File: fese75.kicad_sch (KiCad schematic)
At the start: 166 parts

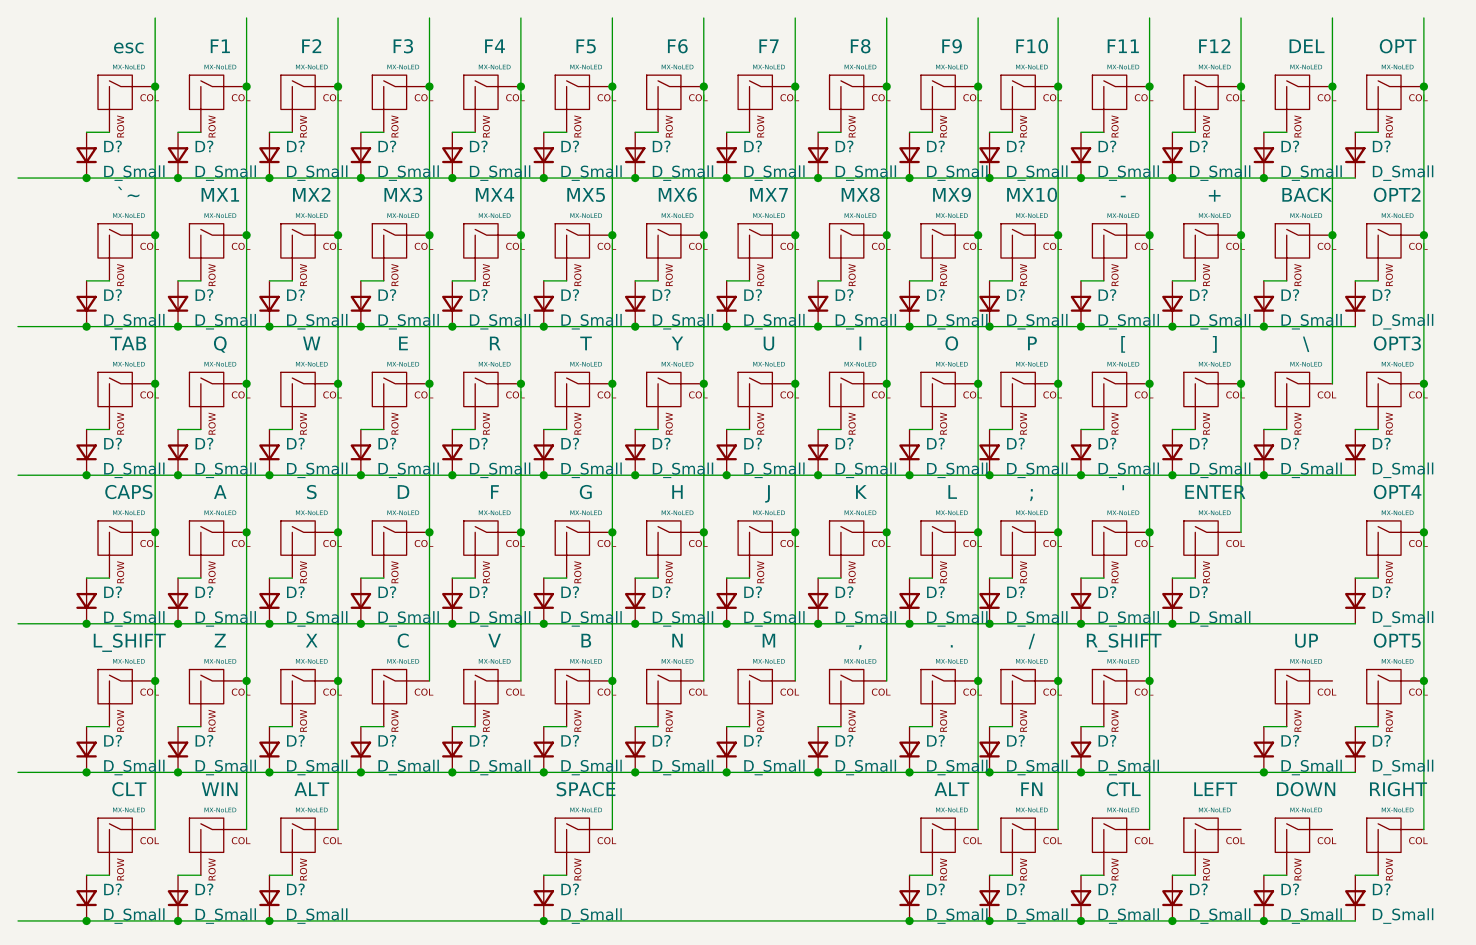
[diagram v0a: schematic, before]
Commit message: quick place component
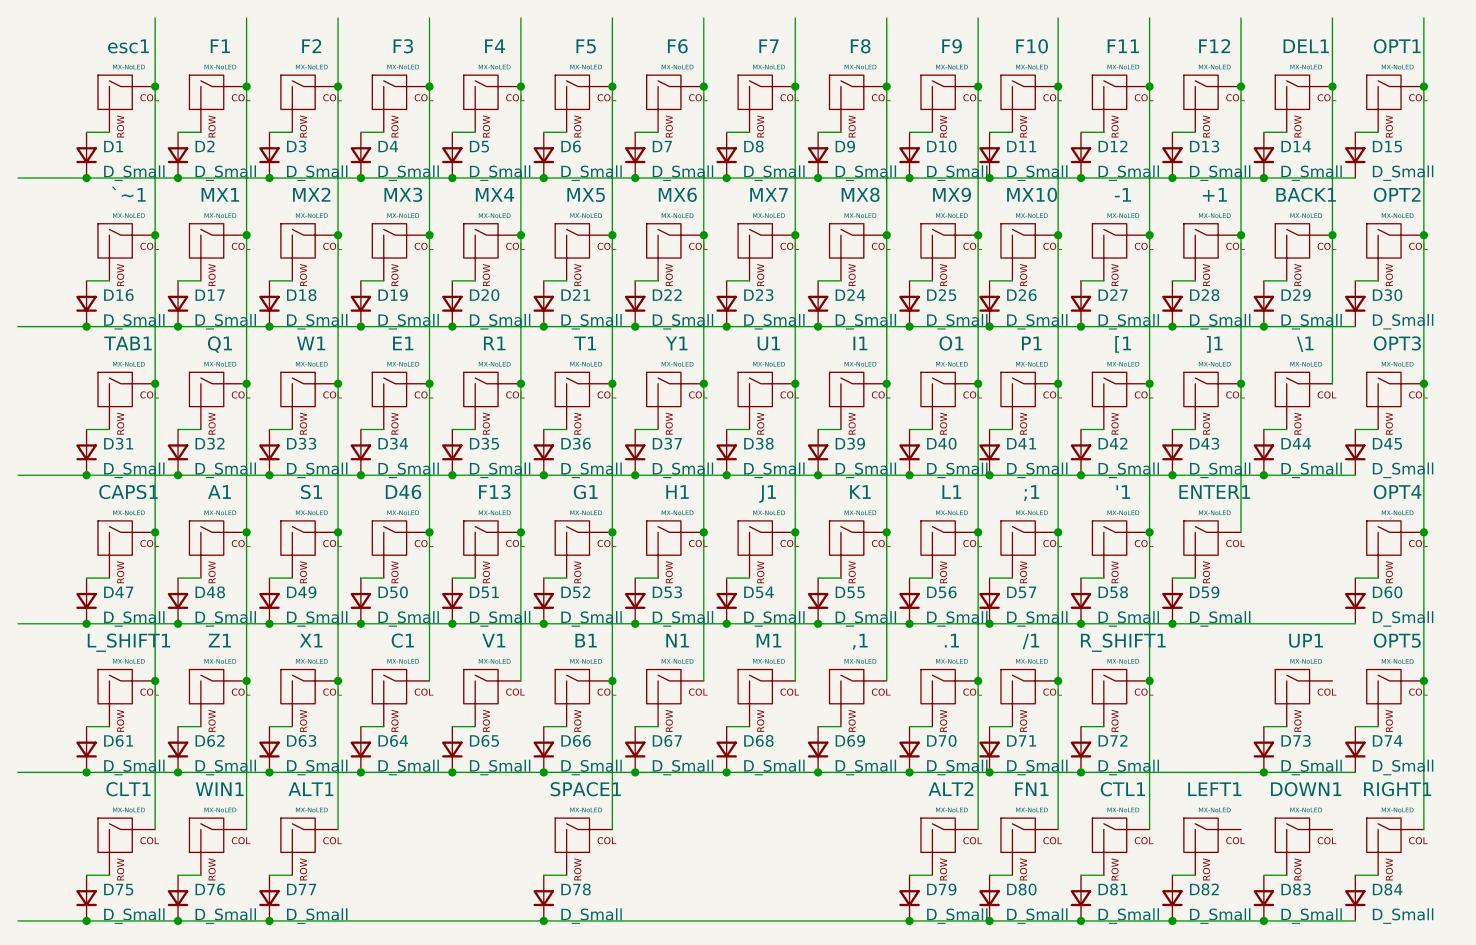
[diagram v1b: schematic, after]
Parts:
- '1: renamed from '; footprint Switch_Keyboard_Kailh:SW_Kailh_Choc_V1_1.00u -> Switch_Keyboard_Kailh:SW_Hotswap_Kailh_1.00u
- ,1: renamed from ,; footprint Mounting_Keyboard_Stabilizer:Stabilizer_Cherry_MX_6.25u -> Switch_Keyboard_Kailh:SW_Hotswap_Kailh_1.00u
- -1: renamed from -; footprint Switch_Keyboard_Kailh:SW_Kailh_Choc_V1_1.00u -> Switch_Keyboard_Kailh:SW_Hotswap_Kailh_1.00u
- .1: renamed from .; footprint Switch_Keyboard_Kailh:SW_Hotswap_Kailh_2.25u -> Switch_Keyboard_Kailh:SW_Hotswap_Kailh_1.00u
- /1: renamed from /; footprint Switch_Keyboard_Kailh:SW_Hotswap_Kailh_2.25u -> Switch_Keyboard_Kailh:SW_Hotswap_Kailh_1.00u
- ;1: renamed from ;; footprint Switch_Keyboard_Kailh:SW_Hotswap_Kailh_2.25u -> Switch_Keyboard_Kailh:SW_Hotswap_Kailh_1.00u
- A1: renamed from A; footprint Switch_Keyboard_Kailh:SW_Kailh_Choc_V1_1.00u -> Switch_Keyboard_Kailh:SW_Hotswap_Kailh_1.00u
- ALT2: renamed from ALT; footprint Switch_Keyboard_Kailh:SW_Hotswap_Kailh_2.25u -> Switch_Keyboard_Kailh:SW_Hotswap_Kailh_1.00u
- B1: renamed from B; footprint Switch_Keyboard_Kailh:SW_Hotswap_Kailh_2.25u -> Switch_Keyboard_Kailh:SW_Hotswap_Kailh_1.00u
- BACK1: renamed from BACK; footprint Mounting_Keyboard_Stabilizer:Stabilizer_Cherry_MX_6.25u -> Switch_Keyboard_Kailh:SW_Hotswap_Kailh_1.00u
- C1: renamed from C; footprint Mounting_Keyboard_Stabilizer:Stabilizer_Cherry_MX_6.25u -> Switch_Keyboard_Kailh:SW_Hotswap_Kailh_1.00u
- CAPS1: renamed from CAPS; footprint Switch_Keyboard_Kailh:SW_Hotswap_Kailh_2.25u -> Switch_Keyboard_Kailh:SW_Hotswap_Kailh_1.00u
- CLT1: renamed from CLT; footprint Switch_Keyboard_Kailh:SW_Hotswap_Kailh_2.25u -> Switch_Keyboard_Kailh:SW_Hotswap_Kailh_1.00u
- CTL1: renamed from CTL; footprint Switch_Keyboard_Kailh:SW_Kailh_Choc_V1_1.00u -> Switch_Keyboard_Kailh:SW_Hotswap_Kailh_1.00u
- D1, D10, D11, D12, D13, D14, D15, D16, D17, D18, D19, D2, D20, D21, D22, D23, D24, D25, D26, D27, D28, D29, D3, D30, D31, D32, D33, D34, D35, D36, D37, D38, D39, D4, D40, D41, D42, D43, D44, D45, D47, D48, D49, D5, D50, D51, D52, D53, D54, D55, D56, D57, D58, D59, D6, D60, D61, D62, D63, D64, D65, D66, D67, D68, D69, D7, D70, D71, D72, D73, D74, D75, D76, D77, D78, D79, D8, D80, D81, D82, D83, D84, D9: renamed from D?; footprint (none) -> Diode_SMD:D_0603_1608Metric_Pad1.05x0.95mm_HandSolder
- D46: renamed from D; footprint Mounting_Keyboard_Stabilizer:Stabilizer_Cherry_MX_6.25u -> Switch_Keyboard_Kailh:SW_Hotswap_Kailh_1.00u
- DEL1: renamed from DEL; footprint Mounting_Keyboard_Stabilizer:Stabilizer_Cherry_MX_6.25u -> Switch_Keyboard_Kailh:SW_Hotswap_Kailh_1.00u
- DOWN1: renamed from DOWN; footprint Mounting_Keyboard_Stabilizer:Stabilizer_Cherry_MX_6.25u -> Switch_Keyboard_Kailh:SW_Hotswap_Kailh_1.00u
- E1: renamed from E; footprint Mounting_Keyboard_Stabilizer:Stabilizer_Cherry_MX_6.25u -> Switch_Keyboard_Kailh:SW_Hotswap_Kailh_1.00u
- F1, F11, F6, MX1, MX6: footprint Switch_Keyboard_Kailh:SW_Kailh_Choc_V1_1.00u -> Switch_Keyboard_Kailh:SW_Hotswap_Kailh_1.00u
- F10, F4, F5, F9, MX10, MX4, MX5, MX9, OPT2, OPT3, OPT4, OPT5: footprint Switch_Keyboard_Kailh:SW_Hotswap_Kailh_2.25u -> Switch_Keyboard_Kailh:SW_Hotswap_Kailh_1.00u
- F13: renamed from F; footprint Switch_Keyboard_Kailh:SW_Hotswap_Kailh_2.25u -> Switch_Keyboard_Kailh:SW_Hotswap_Kailh_1.00u
- F3, F8, MX3, MX8: footprint Mounting_Keyboard_Stabilizer:Stabilizer_Cherry_MX_6.25u -> Switch_Keyboard_Kailh:SW_Hotswap_Kailh_1.00u
- FN1: renamed from FN; footprint Switch_Keyboard_Kailh:SW_Hotswap_Kailh_2.25u -> Switch_Keyboard_Kailh:SW_Hotswap_Kailh_1.00u
- G1: renamed from G; footprint Switch_Keyboard_Kailh:SW_Hotswap_Kailh_2.25u -> Switch_Keyboard_Kailh:SW_Hotswap_Kailh_1.00u
- H1: renamed from H; footprint Switch_Keyboard_Kailh:SW_Kailh_Choc_V1_1.00u -> Switch_Keyboard_Kailh:SW_Hotswap_Kailh_1.00u
- I1: renamed from I; footprint Mounting_Keyboard_Stabilizer:Stabilizer_Cherry_MX_6.25u -> Switch_Keyboard_Kailh:SW_Hotswap_Kailh_1.00u
- K1: renamed from K; footprint Mounting_Keyboard_Stabilizer:Stabilizer_Cherry_MX_6.25u -> Switch_Keyboard_Kailh:SW_Hotswap_Kailh_1.00u
- L1: renamed from L; footprint Switch_Keyboard_Kailh:SW_Hotswap_Kailh_2.25u -> Switch_Keyboard_Kailh:SW_Hotswap_Kailh_1.00u
- L_SHIFT1: renamed from L_SHIFT; footprint Switch_Keyboard_Kailh:SW_Hotswap_Kailh_2.25u -> Switch_Keyboard_Kailh:SW_Hotswap_Kailh_1.00u
- N1: renamed from N; footprint Switch_Keyboard_Kailh:SW_Kailh_Choc_V1_1.00u -> Switch_Keyboard_Kailh:SW_Hotswap_Kailh_1.00u
- O1: renamed from O; footprint Switch_Keyboard_Kailh:SW_Hotswap_Kailh_2.25u -> Switch_Keyboard_Kailh:SW_Hotswap_Kailh_1.00u
- OPT1: renamed from OPT; footprint Switch_Keyboard_Kailh:SW_Hotswap_Kailh_2.25u -> Switch_Keyboard_Kailh:SW_Hotswap_Kailh_1.00u
- P1: renamed from P; footprint Switch_Keyboard_Kailh:SW_Hotswap_Kailh_2.25u -> Switch_Keyboard_Kailh:SW_Hotswap_Kailh_1.00u
- Q1: renamed from Q; footprint Switch_Keyboard_Kailh:SW_Kailh_Choc_V1_1.00u -> Switch_Keyboard_Kailh:SW_Hotswap_Kailh_1.00u
- R1: renamed from R; footprint Switch_Keyboard_Kailh:SW_Hotswap_Kailh_2.25u -> Switch_Keyboard_Kailh:SW_Hotswap_Kailh_1.00u
- RIGHT1: renamed from RIGHT; footprint Switch_Keyboard_Kailh:SW_Hotswap_Kailh_2.25u -> Switch_Keyboard_Kailh:SW_Hotswap_Kailh_1.00u
- R_SHIFT1: renamed from R_SHIFT; footprint Switch_Keyboard_Kailh:SW_Kailh_Choc_V1_1.00u -> Switch_Keyboard_Kailh:SW_Hotswap_Kailh_1.00u
- SPACE1: renamed from SPACE; footprint Switch_Keyboard_Kailh:SW_Kailh_Choc_V1_1.00u -> Switch_Keyboard_Kailh:SW_Hotswap_Kailh_1.00u
- T1: renamed from T; footprint Switch_Keyboard_Kailh:SW_Hotswap_Kailh_2.25u -> Switch_Keyboard_Kailh:SW_Hotswap_Kailh_1.00u
- TAB1: renamed from TAB; footprint Switch_Keyboard_Kailh:SW_Hotswap_Kailh_2.25u -> Switch_Keyboard_Kailh:SW_Hotswap_Kailh_1.00u
- UP1: renamed from UP; footprint Mounting_Keyboard_Stabilizer:Stabilizer_Cherry_MX_6.25u -> Switch_Keyboard_Kailh:SW_Hotswap_Kailh_1.00u
- V1: renamed from V; footprint Switch_Keyboard_Kailh:SW_Hotswap_Kailh_2.25u -> Switch_Keyboard_Kailh:SW_Hotswap_Kailh_1.00u
- WIN1: renamed from WIN; footprint Switch_Keyboard_Kailh:SW_Kailh_Choc_V1_1.00u -> Switch_Keyboard_Kailh:SW_Hotswap_Kailh_1.00u
- Y1: renamed from Y; footprint Switch_Keyboard_Kailh:SW_Kailh_Choc_V1_1.00u -> Switch_Keyboard_Kailh:SW_Hotswap_Kailh_1.00u
- Z1: renamed from Z; footprint Switch_Keyboard_Kailh:SW_Kailh_Choc_V1_1.00u -> Switch_Keyboard_Kailh:SW_Hotswap_Kailh_1.00u
- [1: renamed from [; footprint Switch_Keyboard_Kailh:SW_Kailh_Choc_V1_1.00u -> Switch_Keyboard_Kailh:SW_Hotswap_Kailh_1.00u
- \1: renamed from \; footprint Mounting_Keyboard_Stabilizer:Stabilizer_Cherry_MX_6.25u -> Switch_Keyboard_Kailh:SW_Hotswap_Kailh_1.00u
- `~1: renamed from `~; footprint Switch_Keyboard_Kailh:SW_Hotswap_Kailh_2.25u -> Switch_Keyboard_Kailh:SW_Hotswap_Kailh_1.00u
- esc1: renamed from esc; footprint Switch_Keyboard_Kailh:SW_Hotswap_Kailh_2.25u -> Switch_Keyboard_Kailh:SW_Hotswap_Kailh_1.00u
- renumbered + to +1, ALT to ALT1, ENTER to ENTER1, J to J1, LEFT to LEFT1, M to M1, S to S1, U to U1, W to W1, X to X1, ] to ]1
